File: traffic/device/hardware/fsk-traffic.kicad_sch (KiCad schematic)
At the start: 44 parts, among them J1 JTAG, J2 USB_C, J3 Molex 5569-04A1, J4 Molex 5569-04A1, J5 Molex 5569-04A1, Q1 MMBT5551, Q2 AO3401A, Q3 MMBT5551, Q4 AO3401A, U1 XC6206P332MR, U2 MT3608, U3 STM32F070F6Px, U4 LTV-817S, U5 LTV-817S, Y1 12MHz

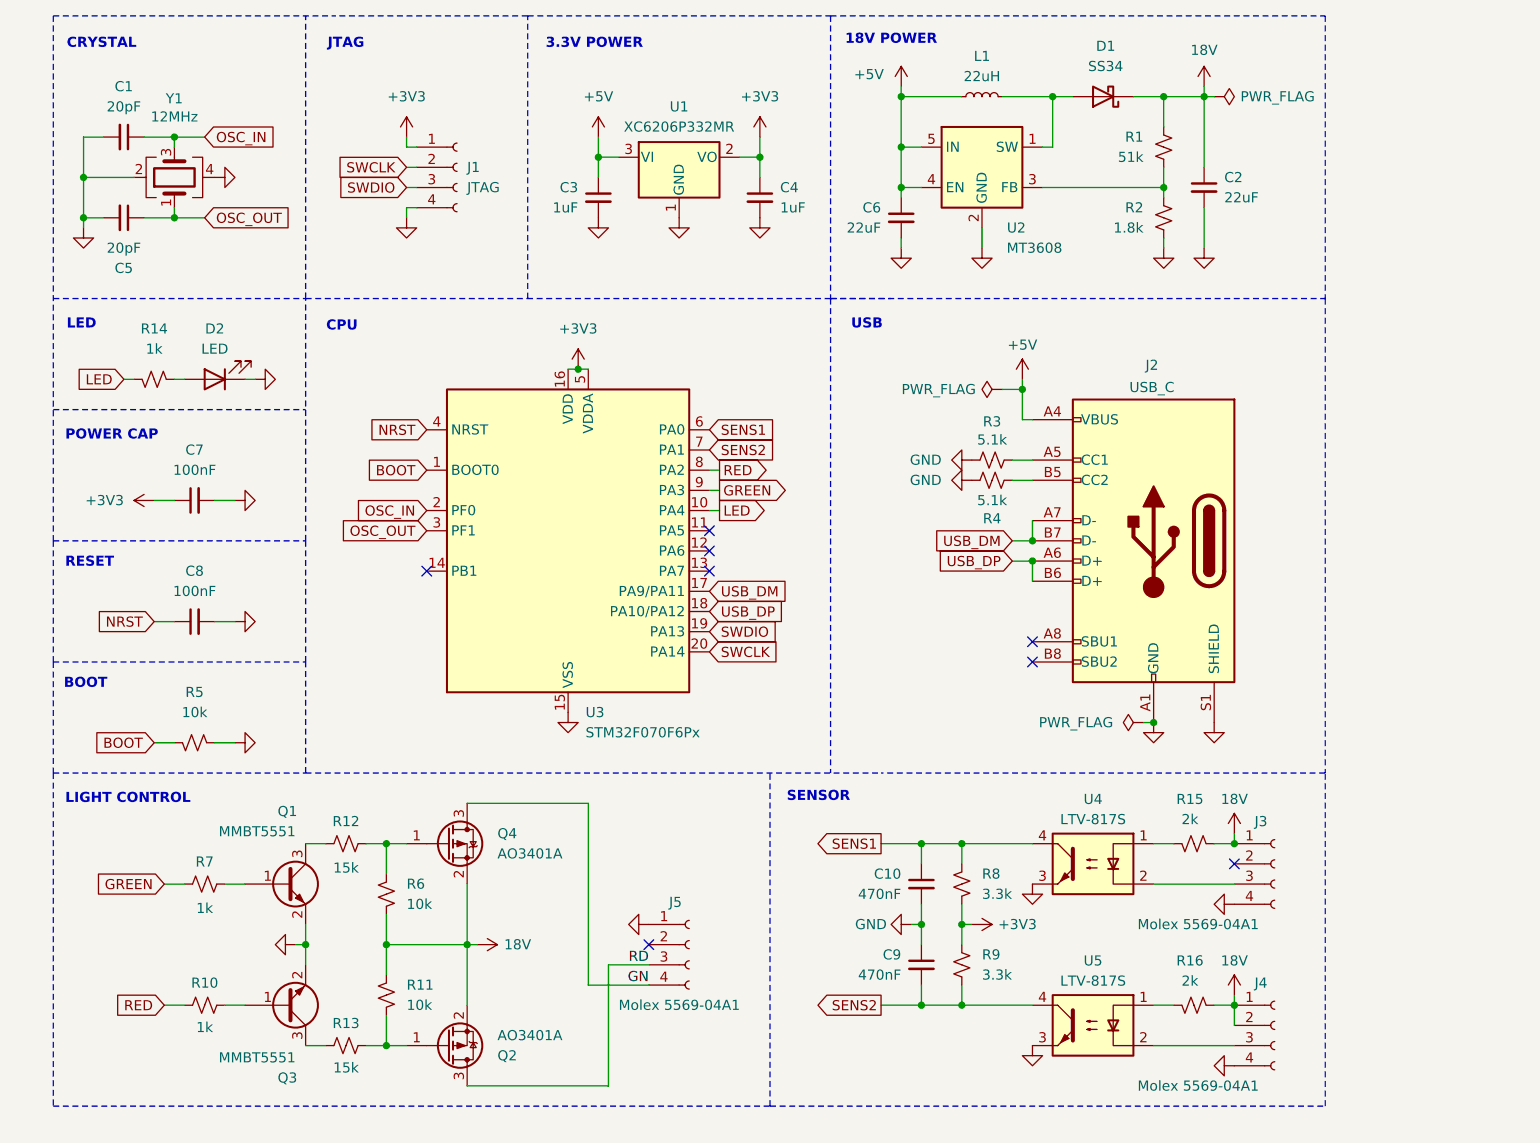
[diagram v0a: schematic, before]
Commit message: impl: schematic and pcb layout
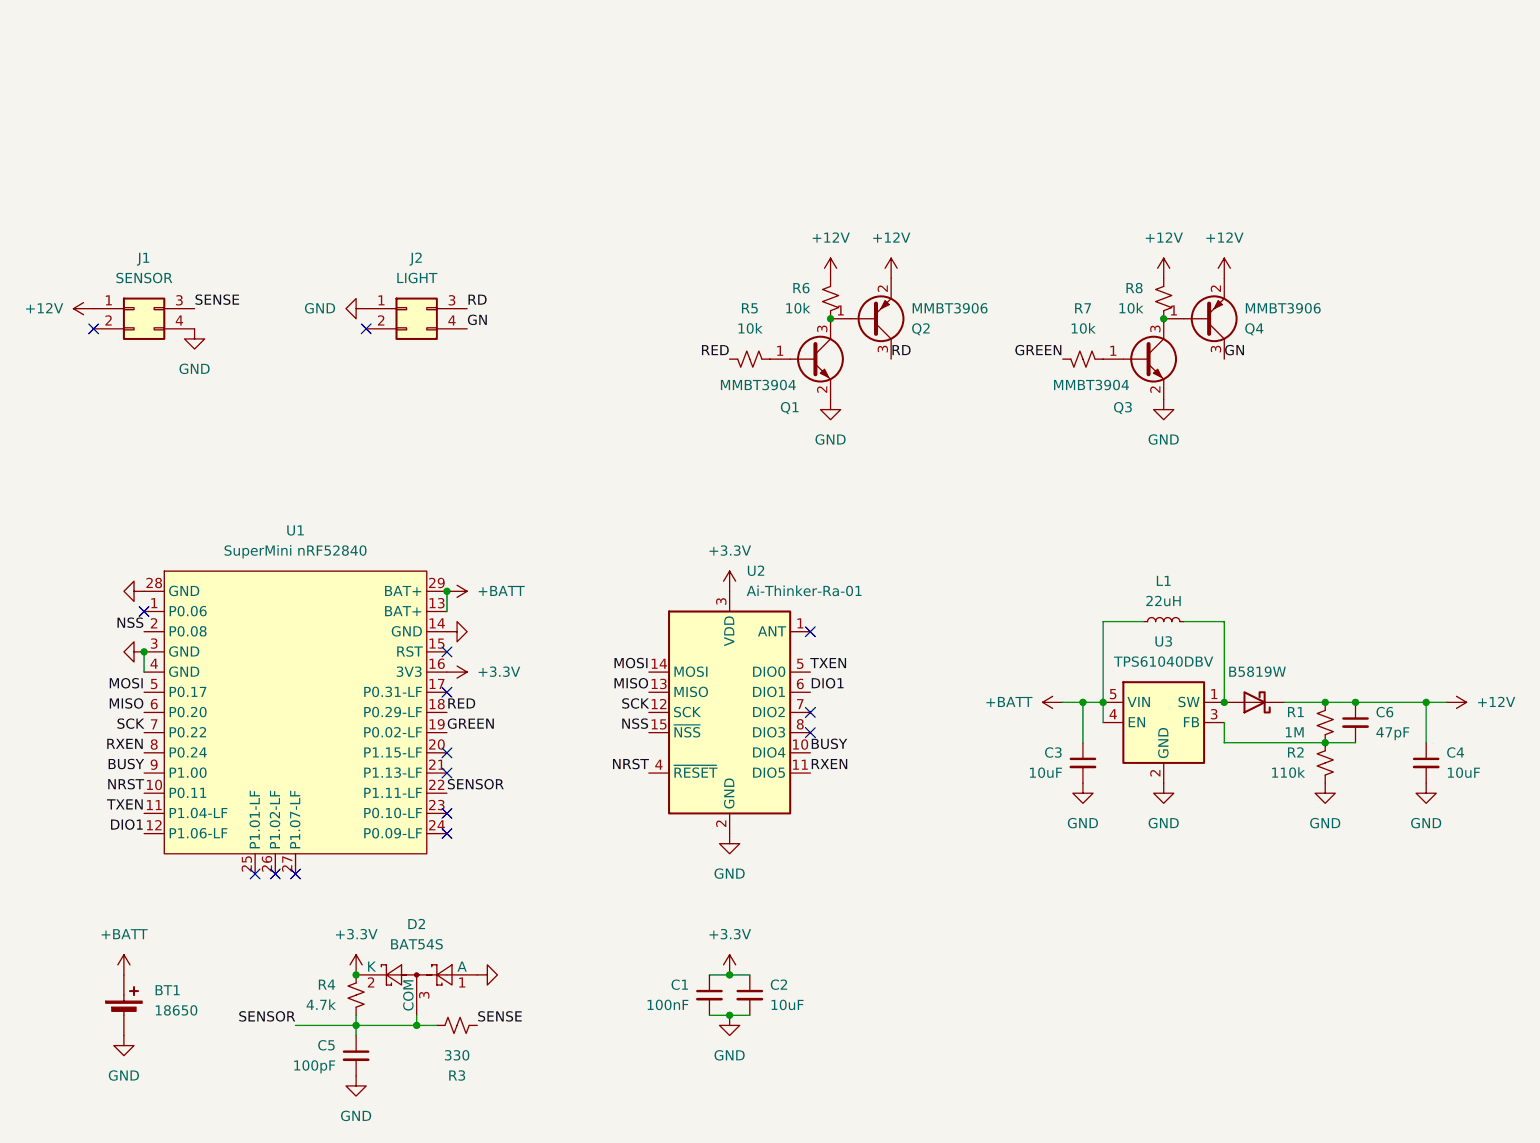
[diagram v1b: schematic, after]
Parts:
- removed C10, C9: 470nF, Capacitor_SMD:C_0603_1608Metric, symbol Device:C_Small
- removed C7, C8: 100nF, Capacitor_SMD:C_0603_1608Metric, symbol Device:C_Small
- removed D1: SS34, Diode_SMD:D_SMA, symbol Diode:SS34
- removed D2: LED, LED_SMD:LED_0603_1608Metric, symbol Device:LED
- removed J1: JTAG, Connector_PinHeader_2.54mm:PinHeader_1x04_P2.54mm_Vertical, symbol Connector:Conn_01x04_Socket
- removed J2: USB_C, Connector_USB:USB_C_Receptacle_GCT_USB4105-xx-A_16P_TopMnt_Horizontal, symbol Connector:USB_C_Receptacle_USB2.0_16P
- removed J3, J4, J5: Molex 5569-04A1, Connector_Molex:Molex_Mini-Fit_Jr_5569-04A1_2x02_P4.20mm_Horizontal, symbol Connector:Conn_01x04_Socket
- removed Q1, Q3: MMBT5551, Package_TO_SOT_SMD:SOT-23, symbol Transistor_BJT:MMBT5551L
- removed Q2, Q4: AO3401A, Package_TO_SOT_SMD:SOT-23, symbol Transistor_FET:AO3401A
- removed R10, R14: 1k, Resistor_SMD:R_0603_1608Metric, symbol Device:R_Small_US
- removed R11: 10k, Resistor_SMD:R_0603_1608Metric, symbol Device:R_Small_US
- removed R12, R13: 15k, Resistor_SMD:R_0603_1608Metric, symbol Device:R_Small_US
- removed R15, R16: 2k, Resistor_SMD:R_0603_1608Metric, symbol Device:R_Small_US
- removed R9: 3.3k, Resistor_SMD:R_0603_1608Metric, symbol Device:R_Small_US
- removed U1: XC6206P332MR, Package_TO_SOT_SMD:SOT-23-3, symbol Regulator_Linear:XC6206PxxxMR
- removed U2: MT3608, Package_TO_SOT_SMD:SOT-23-6, symbol Regulator_Switching:MT3608
- removed U3: STM32F070F6Px, Package_SO:TSSOP-20_4.4x6.5mm_P0.65mm, symbol MCU_ST_STM32F0:STM32F070F6Px
- removed U4, U5: LTV-817S, Package_DIP:SMDIP-4_W9.53mm, symbol Isolator:LTV-817S
- removed Y1: 12MHz, Crystal:Crystal_SMD_3225-4Pin_3.2x2.5mm, symbol Device:Crystal_GND24
- added BT1: 18650, Battery:BatteryHolder_Keystone_1042_1x18650, symbol Device:Battery_Cell
- added D1: B5819W, Diode_SMD:D_SOD-123, symbol Device:D_Schottky
- added D2: BAT54S, Package_TO_SOT_SMD:SOT-23, symbol Diode:BAT54S
- added J1: SENSOR, Connector_Molex:Molex_Mini-Fit_Jr_5569-04A2_2x02_P4.20mm_Horizontal, symbol Connector_Generic:Conn_02x02_Top_Bottom
- added J2: LIGHT, Connector_Molex:Molex_Mini-Fit_Jr_5569-04A2_2x02_P4.20mm_Horizontal, symbol Connector_Generic:Conn_02x02_Top_Bottom
- added Q1, Q3: MMBT3904, Package_TO_SOT_SMD:SOT-23, symbol Transistor_BJT:MMBT3904
- added Q2, Q4: MMBT3906, Package_TO_SOT_SMD:SOT-23, symbol Transistor_BJT:MMBT3906
- added U1: SuperMini nRF52840, lib:SuperMini_NRF52840, symbol SuperMini_NRF52840:SuperMini_nRF52840
- added U2: Ai-Thinker-Ra-01, RF_Module:Ai-Thinker-Ra-01-LoRa, symbol RF_Module:Ai-Thinker-Ra-01
- added U3: TPS61040DBV, Package_TO_SOT_SMD:SOT-23-5, symbol Regulator_Switching:TPS61040DBV
- C1: value 20pF -> 100nF; LCSC C1648 -> C14663
- C2: value 22uF -> 10uF; footprint Capacitor_SMD:C_0805_2012Metric -> Capacitor_SMD:C_0603_1608Metric; LCSC C45783 -> C96446
- C3, C4: value 1uF -> 10uF; LCSC C15849 -> C96446
- C5: value 20pF -> 100pF; LCSC C1648 -> C14858
- C6: value 22uF -> 47pF; footprint Capacitor_SMD:C_0805_2012Metric -> Capacitor_SMD:C_0603_1608Metric; LCSC C45783 -> C1671
- L1: footprint Inductor_SMD:L_Changjiang_FXL0630 -> Inductor_SMD:L_Sunlord_MWSA0603S; LCSC C177244 -> (none)
- R1: value 51k -> 1M; LCSC C23196 -> C22935
- R2: value 1.8k -> 110k; LCSC C4177 -> C25805
- R3: value 5.1k -> 330; LCSC C23186 -> C23138
- R4: value 5.1k -> 4.7k; LCSC C23186 -> C23162
- R7: value 1k -> 10k; LCSC C21190 -> C25804
- R8: value 3.3k -> 10k; LCSC C22978 -> C25804
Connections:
- net BOOT is gone; now on net RED: R5.2
- net OSC_IN is gone; now on net +3.3V: C1.1
- net OSC_OUT is gone; now on net SENSOR: C5.1
- net SENS1 is gone; now on net +12V: R8.1
- net GN: now also J2.4 (Pin_4), Q4.3 (C)
- net GND: now also BT1.2 (-), D2.1 (A), J1.4 (Pin_4), J2.1 (Pin_1), Q1.2 (E), Q3.2 (E), U1.14 (GND), U1.28 (GND), U1.3 (GND), U1.4 (GND), U2.16 (GND), U2.2 (GND), U2.9 (GND), U3.2 (GND); no longer C6.2, R3.1, R4.1, R5.1
- net GREEN: now also U1.19 (P0.02-LF)
- net NRST: now also U1.10 (P0.11), U2.4 (~{RESET})
- net RD: now also J2.3 (Pin_3), Q2.3 (C)
- net RED: now also U1.18 (P0.29-LF)
- net SENSOR: now reaches R3.2
- net SENSOR: now also R4.1, D2.3 (COM), U1.22 (P1.11-LF)
- net +3.3V: now reaches R4.2
- net +3.3V: now also C2.1, D2.2 (K), U1.16 (3V3), U2.3 (VDD)
- net at R7.1: now also Q3.1 (B)
- net at L1.2: now also D1.2 (A), U3.1 (SW)
- net +12V: now reaches R6.1
- net +12V: now also C4.1, C6.1, R1.1, D1.1 (K), J1.1 (Pin_1), Q2.2 (E), Q4.2 (E)
- net at R1.2, R2.1: now also C6.2, U3.3 (FB)
- net +3V3: no longer names the net of R8.2
- net +3V3: now also Q3.3 (C), Q4.1 (B); no longer C4.1
- net +5V renamed +BATT
- net +BATT: now also BT1.1 (+), U1.13 (BAT+), U1.29 (BAT+), U3.4 (EN), U3.5 (VIN); no longer C6.1
- removed net 18V: C2.1, R1.1, R6.2
- new net: Q1.3 (C), Q2.1 (B), R6.2
- new net: Q1.1 (B), R5.1
- new net BUSY: U1.9 (P1.00), U2.10 (DIO4)
- new net DIO1: U1.12 (P1.06-LF), U2.6 (DIO1)
- new net MISO: U1.6 (P0.20), U2.13 (MISO)
- new net MOSI: U1.5 (P0.17), U2.14 (MOSI)
- new net NSS: U1.2 (P0.08), U2.15 (~{NSS})
- new net RXEN: U1.8 (P0.24), U2.11 (DIO5)
- new net SCK: U1.7 (P0.22), U2.12 (SCK)
- new net SENSE: J1.3 (Pin_3), R3.1
- new net TXEN: U1.11 (P1.04-LF), U2.5 (DIO0)
- no-connect marks 8 -> 15
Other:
- note removed: "18V POWER"
- note removed: "3.3V POWER"
- note removed: "BOOT"
- note removed: "CPU"
- note removed: "CRYSTAL"
- note removed: "JTAG"
- note removed: "LED"
- note removed: "LIGHT CONTROL"
- note removed: "POWER CAP"
- note removed: "RESET"
- note removed: "SENSOR"
- note removed: "USB"
